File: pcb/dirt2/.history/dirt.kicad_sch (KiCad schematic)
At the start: 8 parts, among them P1 USB_C_Plug_USB2.0

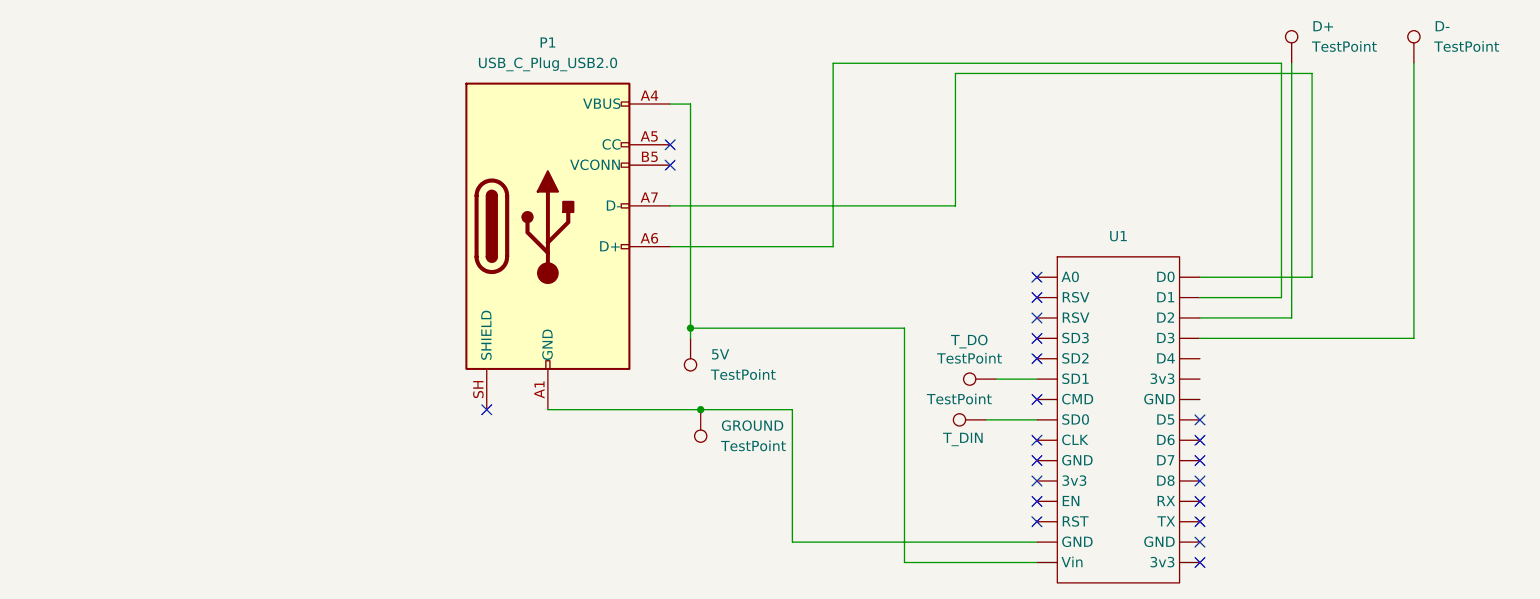
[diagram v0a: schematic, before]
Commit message: i created some edits and added the zine
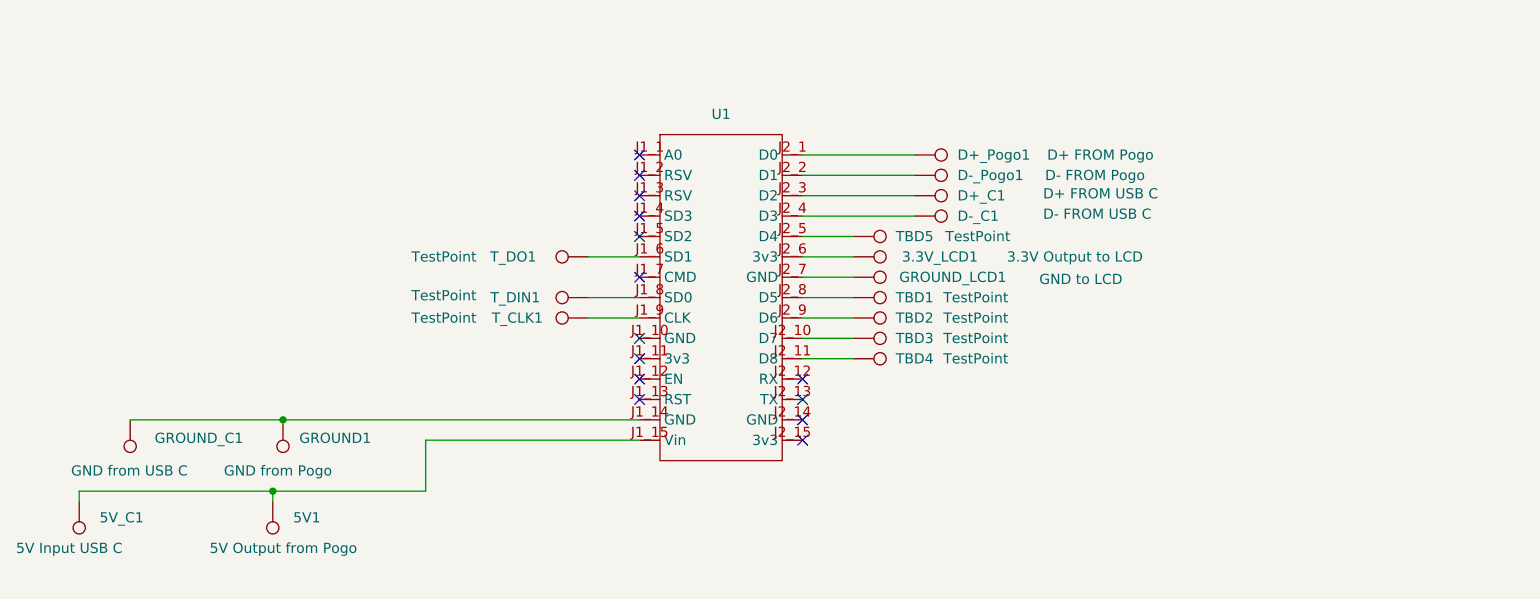
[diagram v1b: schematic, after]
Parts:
- removed P1: USB_C_Plug_USB2.0, symbol Connector:USB_C_Plug_USB2.0
- added 3.3V_LCD1: 3.3V Output to LCD, TestPoint:TestPoint_THTPad_D1.0mm_Drill0.5mm, symbol Connector:TestPoint
- added 5V_C1: 5V Input USB C, TestPoint:TestPoint_THTPad_D1.0mm_Drill0.5mm, symbol Connector:TestPoint
- added D+_Pogo1: D+ FROM Pogo, TestPoint:TestPoint_THTPad_D1.0mm_Drill0.5mm, symbol Connector:TestPoint
- added D-_Pogo1: D- FROM Pogo, TestPoint:TestPoint_THTPad_D1.0mm_Drill0.5mm, symbol Connector:TestPoint
- added GROUND_C1: GND from USB C, TestPoint:TestPoint_THTPad_D1.0mm_Drill0.5mm, symbol Connector:TestPoint
- added GROUND_LCD1: GND to LCD, TestPoint:TestPoint_THTPad_D1.0mm_Drill0.5mm, symbol Connector:TestPoint
- added TBD1, TBD2, TBD3, TBD4, TBD5: TestPoint, symbol Connector:TestPoint
- added T_CLK1: TestPoint, TestPoint:TestPoint_THTPad_D1.0mm_Drill0.5mm, symbol Connector:TestPoint
- 5V1: renamed from 5V; value TestPoint -> 5V Output from Pogo; footprint (none) -> TestPoint:TestPoint_THTPad_D1.0mm_Drill0.5mm
- D+_C1: renamed from D+; value TestPoint -> D+ FROM USB C; footprint (none) -> TestPoint:TestPoint_THTPad_D1.0mm_Drill0.5mm
- D-_C1: renamed from D-; value TestPoint -> D- FROM USB C; footprint (none) -> TestPoint:TestPoint_THTPad_D1.0mm_Drill0.5mm
- GROUND1: renamed from GROUND; value TestPoint -> GND from Pogo; footprint (none) -> TestPoint:TestPoint_THTPad_D1.0mm_Drill0.5mm
- T_DIN1: renamed from T_DIN; footprint (none) -> TestPoint:TestPoint_THTPad_D1.0mm_Drill0.5mm
- T_DO1: renamed from T_DO; footprint (none) -> TestPoint:TestPoint_THTPad_D1.0mm_Drill0.5mm
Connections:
- net at GROUND1.1: now also U1.J1_14 (GND), GROUND_C1.1; no longer U1. (3v3)
- net at D-_C1.1: now also U1.J2_4 (D3); no longer U1. (3v3)
- net at T_DIN1.1: now also U1.J1_8 (SD0); no longer U1. (3v3)
- net at 5V1.1: now also U1.J1_15 (Vin), 5V_C1.1; no longer U1. (3v3)
- net at T_DO1.1: now also U1.J1_6 (SD1); no longer U1. (3v3)
- net at D+_C1.1: now also U1.J2_3 (D2); no longer U1. (3v3)
- new net: T_CLK1.1, U1.J1_9 (CLK)
- new net: D+_Pogo1.1, U1.J2_1 (D0)
- new net: TBD3.1, U1.J2_10 (D7)
- new net: TBD4.1, U1.J2_11 (D8)
- new net: D-_Pogo1.1, U1.J2_2 (D1)
- new net: TBD5.1, U1.J2_5 (D4)
- new net: 3.3V_LCD1.1, U1.J2_6 (3v3)
- new net: GROUND_LCD1.1, U1.J2_7 (GND)
- new net: TBD1.1, U1.J2_8 (D5)
- new net: TBD2.1, U1.J2_9 (D6)
- no-connect marks 22 -> 14
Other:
- moved on the sheet: 5V1, D+_C1, D-_C1, GROUND1, T_DIN1, T_DO1
